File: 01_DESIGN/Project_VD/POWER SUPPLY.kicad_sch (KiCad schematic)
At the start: 22 parts, among them J1 12V, J2 USB_B_Micro, U1 LM1117MP-3.3, U2 LM2596S-5

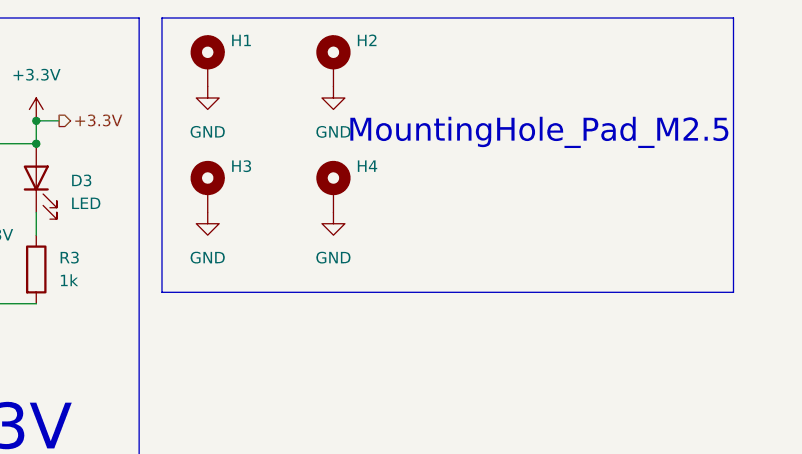
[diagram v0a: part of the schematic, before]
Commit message: update 21/06/2026
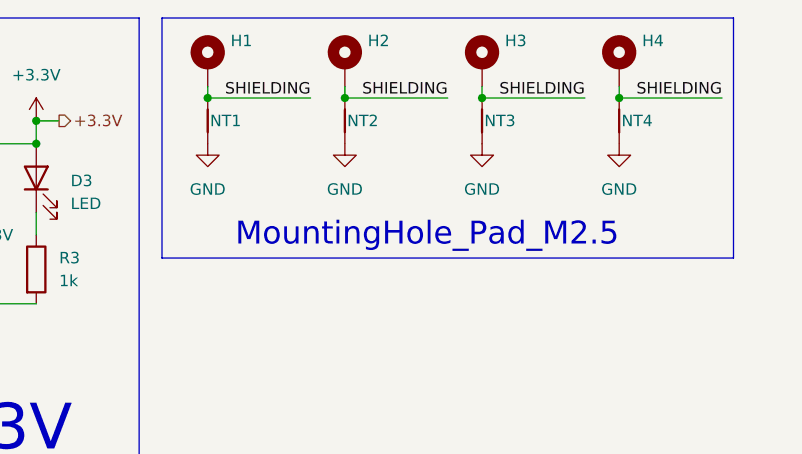
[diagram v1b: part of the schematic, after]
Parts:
- added NT1, NT2, NT3, NT4: NetTie_2, NetTie:NetTie-2_SMD_Pad0.5mm, symbol Device:NetTie_2
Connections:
- net GND: now also NT1.1, NT2.1, NT3.1, NT4.1; no longer H1.1, H2.1, H3.1, H4.1
- new net SHIELDING: H1.1, H2.1, H3.1, H4.1, NT1.2, NT2.2, NT3.2, NT4.2
